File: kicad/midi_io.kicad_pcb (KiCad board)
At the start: 2 copper layers, 35.6 x 41.4 mm, 10 parts, among them J1 MIDI Out, J2 MIDI In, J3 Conn_01x04, U1 6N138

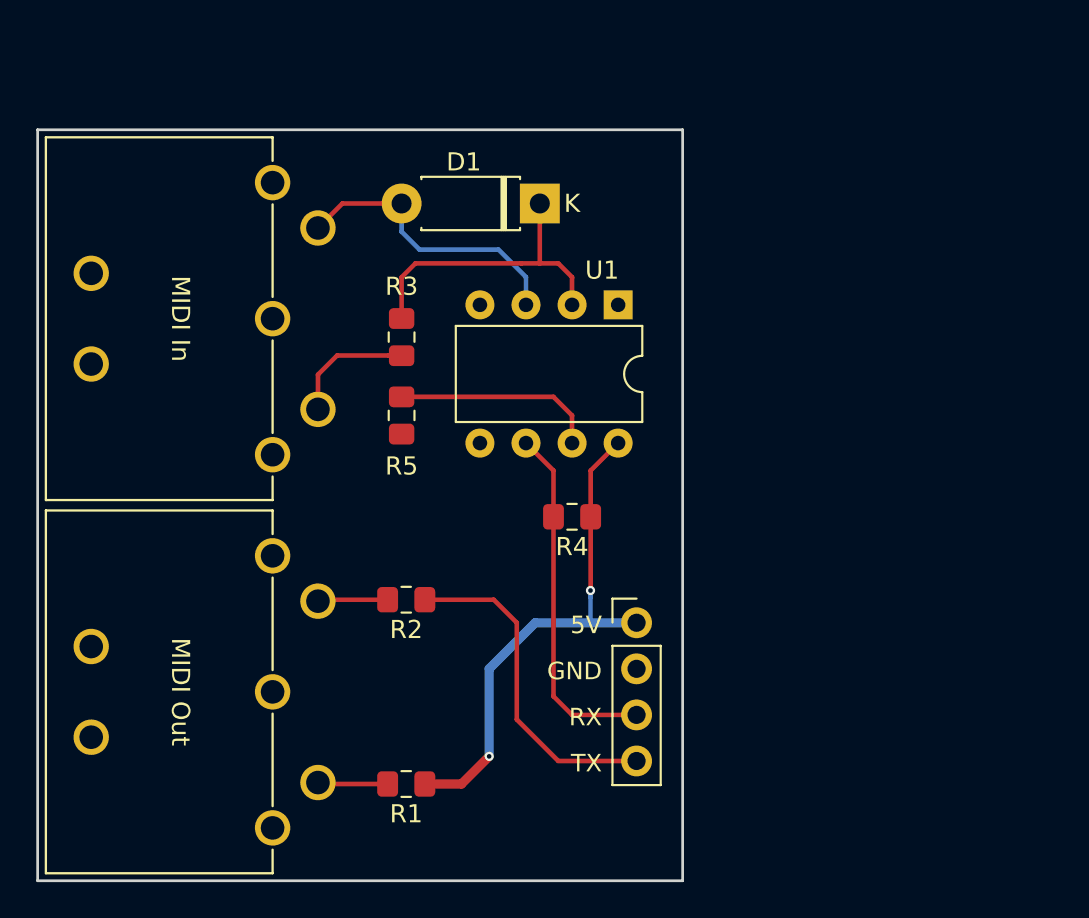
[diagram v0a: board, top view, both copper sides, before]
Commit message: Misc
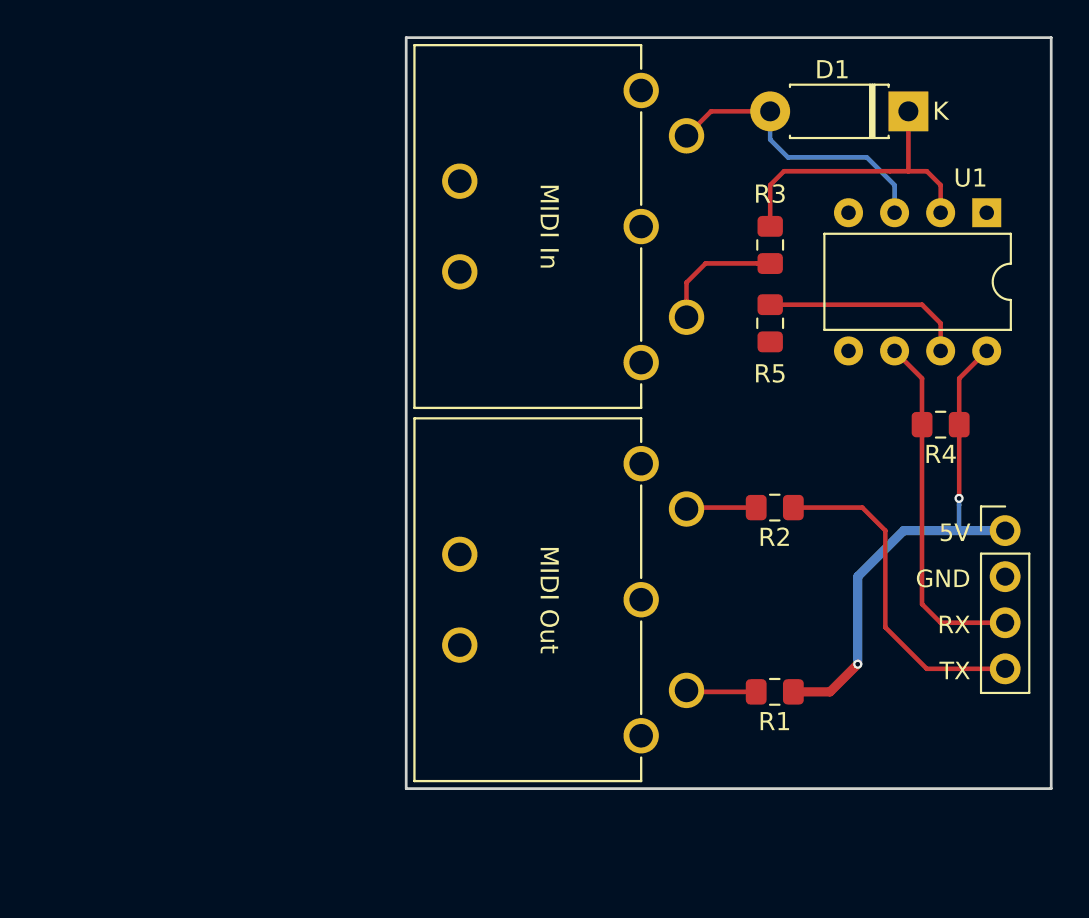
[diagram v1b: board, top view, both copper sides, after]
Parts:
- moved R4 20.9 mm to (160.8, 100.7)
- moved D1 20.9 mm to (159.0, 83.4)
- moved J1 20.9 mm to (144.3, 110.4)
- moved J2 20.9 mm to (144.3, 89.8)
- moved J3 20.9 mm to (164.3, 106.6)
- moved R1 20.9 mm to (151.6, 115.4)
- moved R2 20.9 mm to (151.6, 105.3)
- moved R3 20.9 mm to (151.4, 90.8)
- moved R5 20.9 mm to (151.4, 95.1)
- moved U1 20.9 mm to (163.3, 89.0)
